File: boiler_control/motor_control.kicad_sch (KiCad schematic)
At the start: 12 parts, among them U4 MOC3162M

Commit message: Replace max3856 with SSOP package; replace all 0201 res/cap packages with 0603
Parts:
- R10, R14: footprint Resistor_SMD:R_1206_3216Metric_Pad1.30x1.75mm_HandSolder -> Resistor_SMD:R_0603_1608Metric_Pad0.98x0.95mm_HandSolder
- U4: footprint Package_DIP:DIP-6_W7.62mm_SMDSocket_SmallPads -> Package_DIP:DIP-6_W8.89mm_SMDSocket_LongPads
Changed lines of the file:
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@@
       (effects (font (size 1.27 1.27)) (justify right))
     )
-    (property "Footprint" "Resistor_SMD:R_1206_3216Metric_Pad1.30x1.75mm_HandSolder" (at 52.578 54.61 90)
+    (property "Footprint" "Resistor_SMD:R_0603_1608Metric_Pad0.98x0.95mm_HandSolder" (at 52.578 54.61 90)
       (effects (font (size 1.27 1.27)) hide)
     )
@@
       (effects (font (size 1.27 1.27)))
     )
-    (property "Footprint" "Package_DIP:DIP-6_W7.62mm_SMDSocket_SmallPads" (at 72.39 55.88 0)
+    (property "Footprint" "Package_DIP:DIP-6_W8.89mm_SMDSocket_LongPads" (at 72.39 55.88 0)
       (effects (font (size 1.27 1.27) italic) (justify left) hide)
     )
@@
       (effects (font (size 1.27 1.27)))
     )
-    (property "Footprint" "Resistor_SMD:R_1206_3216Metric_Pad1.30x1.75mm_HandSolder" (at 60.96 50.038 90)
+    (property "Footprint" "Resistor_SMD:R_0603_1608Metric_Pad0.98x0.95mm_HandSolder" (at 60.96 50.038 90)
       (effects (font (size 1.27 1.27)) hide)
     )

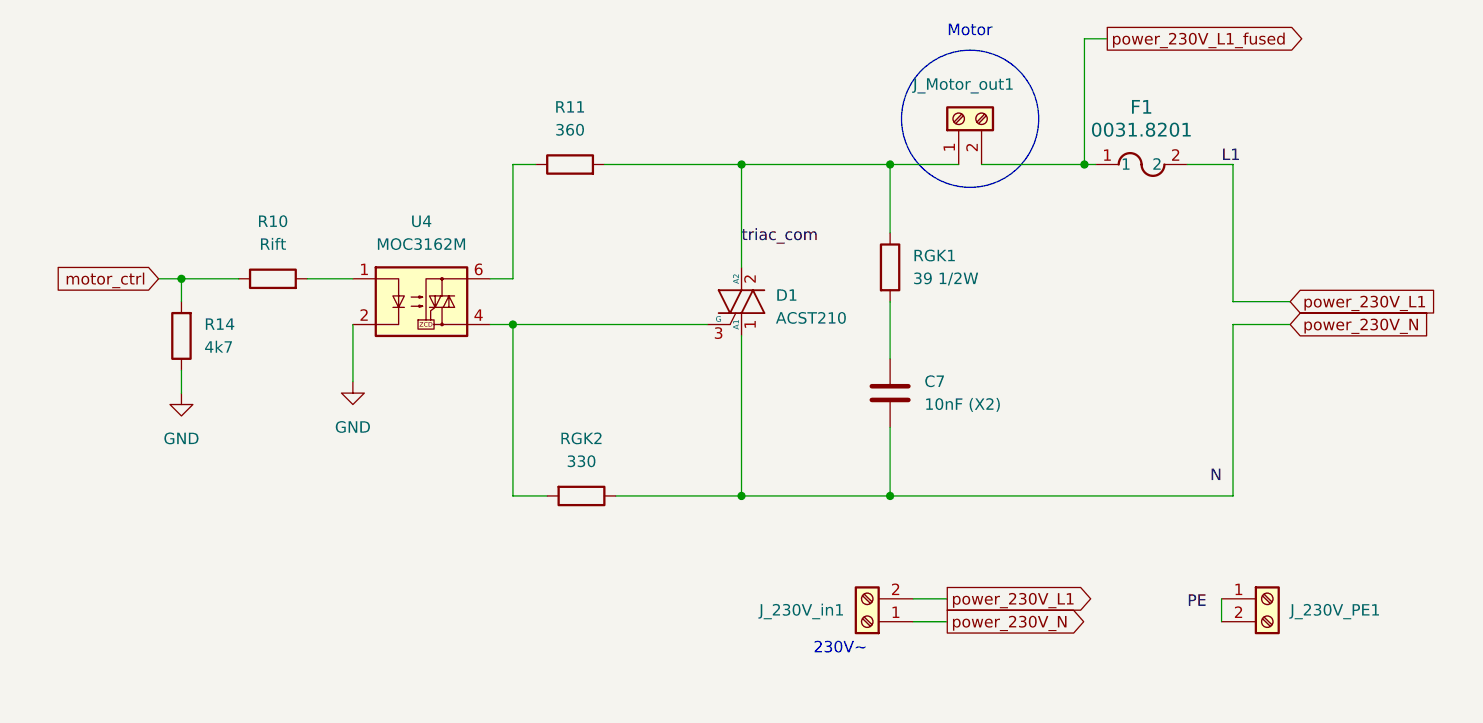
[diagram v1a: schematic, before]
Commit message: Updating to v1.4 - pushed to order
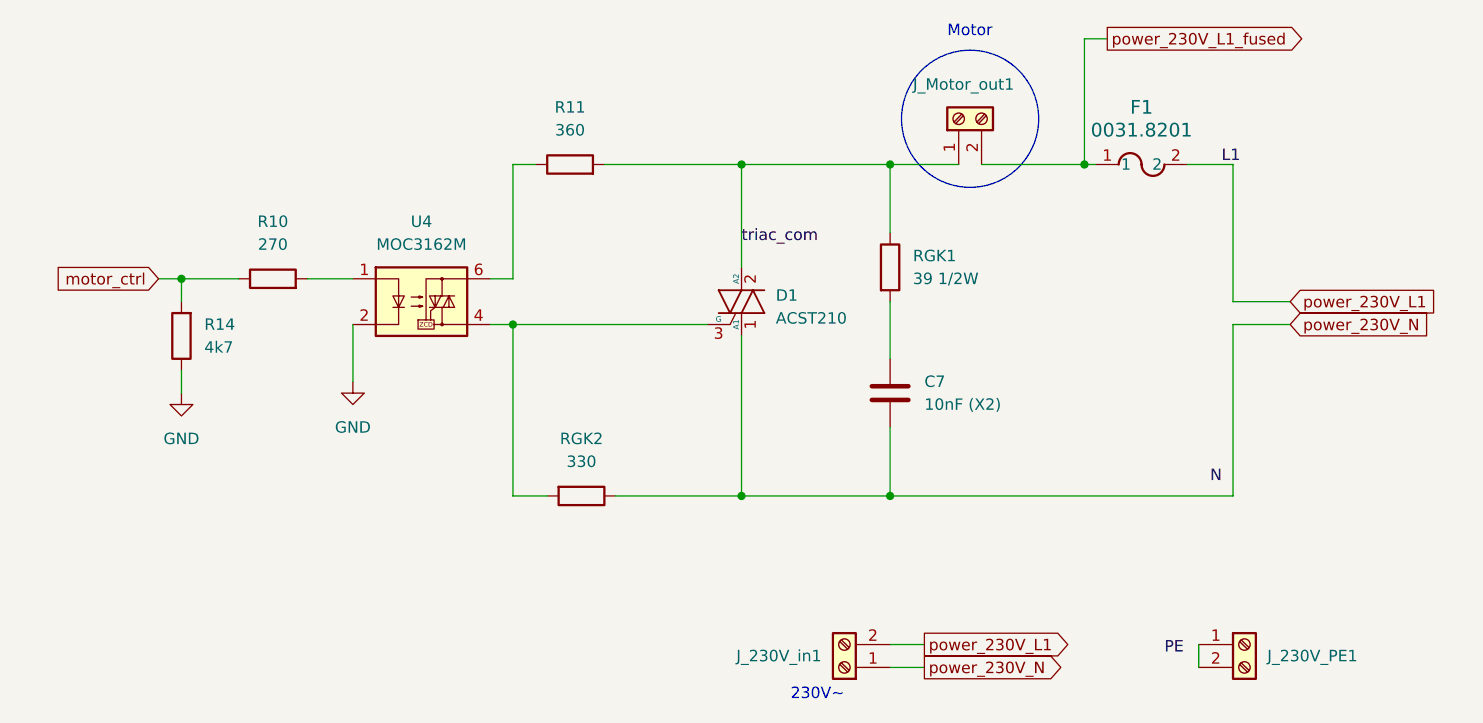
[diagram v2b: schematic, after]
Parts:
- F1: footprint Fuse:Fuseholder_Clip-5x20mm_Schurter_CQM_Inline_P20.60x5.00mm_D1.00mm_Horizontal -> Fuse:Fuseholder_Clip-5x20mm_Littelfuse_445-030_Inline_P20.50x5.20mm_D1.30mm_Horizontal
- R10: value Rift -> 270
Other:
- moved on the sheet: J_230V_PE1, J_230V_in1
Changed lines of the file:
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@@
     (stroke (width 0) (type default))
   )
-  (wire (pts (xy 132.08 83.82) (xy 135.89 83.82))
+  (wire (pts (xy 129.54 88.9) (xy 133.35 88.9))
     (stroke (width 0) (type default))
   )
@@
     (stroke (width 0) (type default))
   )
-  (wire (pts (xy 132.08 86.36) (xy 135.89 86.36))
+  (wire (pts (xy 129.54 91.44) (xy 133.35 91.44))
     (stroke (width 0) (type default))
   )
@@
     (stroke (width 0) (type default))
   )
-  (wire (pts (xy 166.37 83.82) (xy 166.37 86.36))
+  (wire (pts (xy 163.83 88.9) (xy 163.83 91.44))
     (stroke (width 0) (type default))
   )
@@
     (effects (font (size 1.27 1.27)) (justify left bottom))
   )
-  (text "230V~" (at 127 90.17 0)
+  (text "230V~" (at 124.46 95.25 0)
     (effects (font (size 1.27 1.27)) (justify right bottom))
   )
-  (label "PE" (at 162.56 85.09 0) (fields_autoplaced)
+  (label "PE" (at 160.02 90.17 0) (fields_autoplaced)
     (effects (font (size 1.27 1.27)) (justify left bottom))
   )
@@
     )
   )
-  (global_label "power_230V_L1" (shape output) (at 135.89 83.82 0) (fields_autoplaced)
+  (global_label "power_230V_L1" (shape output) (at 133.35 88.9 0) (fields_autoplaced)
     (effects (font (size 1.27 1.27)) (justify left))
-    (property "Intersheetrefs" "${INTERSHEET_REFS}" (at 153.2684 83.82 0)
-      (effects (font (size 1.27 1.27)) (justify left) hide)
-    )
-  )
-  (global_label "power_230V_N" (shape output) (at 135.89 86.36 0) (fields_autoplaced)
+    (property "Intersheetrefs" "${INTERSHEET_REFS}" (at 150.7284 88.9 0)
+      (effects (font (size 1.27 1.27)) (justify left) hide)
+    )
+  )
+  (global_label "power_230V_N" (shape output) (at 133.35 91.44 0) (fields_autoplaced)
     (effects (font (size 1.27 1.27)) (justify left))
-    (property "Intersheetrefs" "${INTERSHEET_REFS}" (at 152.3613 86.36 0)
+    (property "Intersheetrefs" "${INTERSHEET_REFS}" (at 149.8213 91.44 0)
       (effects (font (size 1.27 1.27)) (justify left) hide)
     )
@@
     )
   )
-  (symbol (lib_id "Connector:Screw_Terminal_01x02") (at 171.45 83.82 0) (unit 1)
+  (symbol (lib_id "Connector:Screw_Terminal_01x02") (at 168.91 88.9 0) (unit 1)
     (in_bom yes) (on_board yes) (dnp no)
-    (property "Reference" "J_230V_PE1" (at 173.99 85.09 0)
-      (effects (font (size 1.27 1.27)) (justify left))
-    )
-    (property "Value" "Screw_Terminal_01x02" (at 173.99 86.36 0)
-      (effects (font (size 1.27 1.27)) (justify left) hide)
-    )
-    (property "Footprint" "TerminalBlock:TerminalBlock_bornier-2_P5.08mm" (at 171.45 83.82 0)
-      (effects (font (size 1.27 1.27)) hide)
-    )
-    (property "Datasheet" "~" (at 171.45 83.82 0)
+    (property "Reference" "J_230V_PE1" (at 171.45 90.17 0)
+      (effects (font (size 1.27 1.27)) (justify left))
+    )
+    (property "Value" "Screw_Terminal_01x02" (at 171.45 91.44 0)
+      (effects (font (size 1.27 1.27)) (justify left) hide)
+    )
+    (property "Footprint" "TerminalBlock:TerminalBlock_bornier-2_P5.08mm" (at 168.91 88.9 0)
+      (effects (font (size 1.27 1.27)) hide)
+    )
+    (property "Datasheet" "~" (at 168.91 88.9 0)
       (effects (font (size 1.27 1.27)) hide)
     )
@@
     )
   )
-  (symbol (lib_id "Connector:Screw_Terminal_01x02") (at 127 86.36 180) (unit 1)
+  (symbol (lib_id "Connector:Screw_Terminal_01x02") (at 124.46 91.44 180) (unit 1)
     (in_bom yes) (on_board yes) (dnp no)
-    (property "Reference" "J_230V_in1" (at 124.46 85.09 0)
-      (effects (font (size 1.27 1.27)) (justify left))
-    )
-    (property "Value" "Screw_Terminal_01x02" (at 124.46 83.82 0)
-      (effects (font (size 1.27 1.27)) (justify left) hide)
-    )
-    (property "Footprint" "TerminalBlock:TerminalBlock_bornier-2_P5.08mm" (at 127 86.36 0)
-      (effects (font (size 1.27 1.27)) hide)
-    )
-    (property "Datasheet" "~" (at 127 86.36 0)
+    (property "Reference" "J_230V_in1" (at 121.92 90.17 0)
+      (effects (font (size 1.27 1.27)) (justify left))
+    )
+    (property "Value" "Screw_Terminal_01x02" (at 121.92 88.9 0)
+      (effects (font (size 1.27 1.27)) (justify left) hide)
+    )
+    (property "Footprint" "TerminalBlock:TerminalBlock_bornier-2_P5.08mm" (at 124.46 91.44 0)
+      (effects (font (size 1.27 1.27)) hide)
+    )
+    (property "Datasheet" "~" (at 124.46 91.44 0)
       (effects (font (size 1.27 1.27)) hide)
     )
@@
       (effects (font (size 1.524 1.524)))
     )
-    (property "Footprint" "Fuse:Fuseholder_Clip-5x20mm_Schurter_CQM_Inline_P20.60x5.00mm_D1.00mm_Horizontal" (at 152.4 35.56 0)
+    (property "Footprint" "Fuse:Fuseholder_Clip-5x20mm_Littelfuse_445-030_Inline_P20.50x5.20mm_D1.30mm_Horizontal" (at 152.4 35.56 0)
       (effects (font (size 1.27 1.27) italic) hide)
     )
@@
       (effects (font (size 1.27 1.27)))
     )
-    (property "Value" "Rift" (at 60.96 44.45 90)
-      (effects (font (size 1.27 1.27)))
-    )
+    (property "Value" "270" (at 60.96 44.45 90)
+      (effects (font (size 1.27 1.27)))
+    )
